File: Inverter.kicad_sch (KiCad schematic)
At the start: 45 parts, among them Q2 BSC022N04LSATMA1, Q3 BSC022N04LSATMA1, Q4 BSC022N04LSATMA1, Q5 BSC022N04LSATMA1, Q6 BSC022N04LSATMA1, Q7 BSC022N04LSATMA1, U4 TMC6140, U5 TSC2011, U6 TSC2011

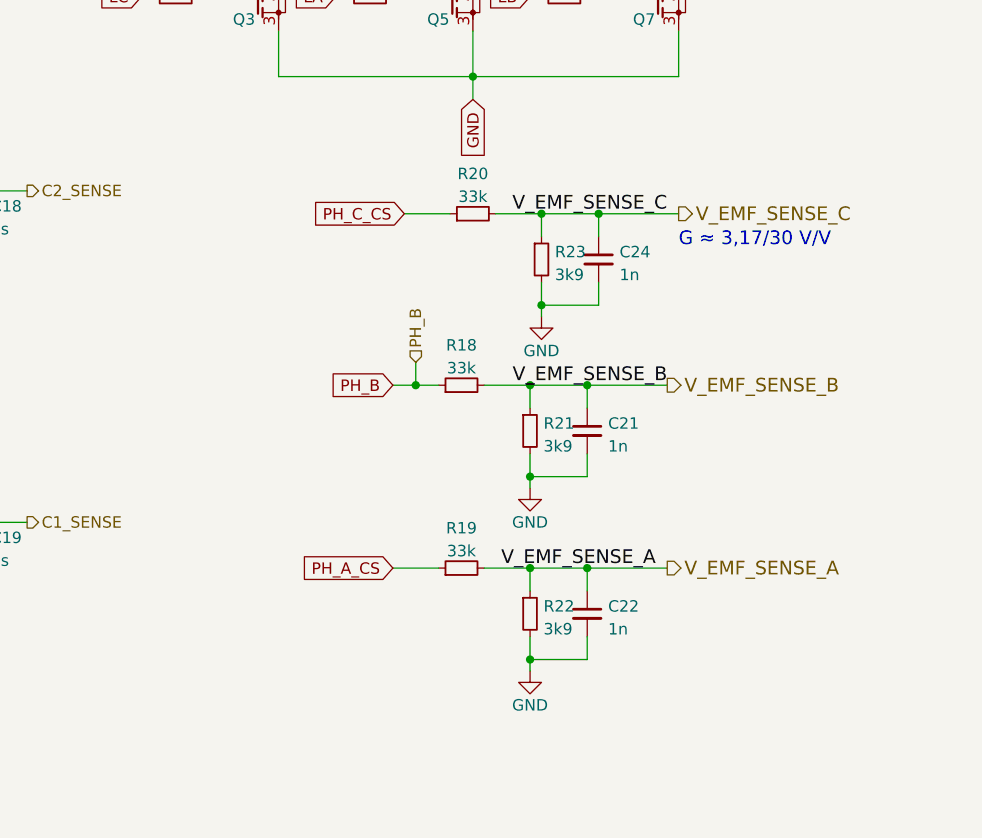
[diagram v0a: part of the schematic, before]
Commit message: layout
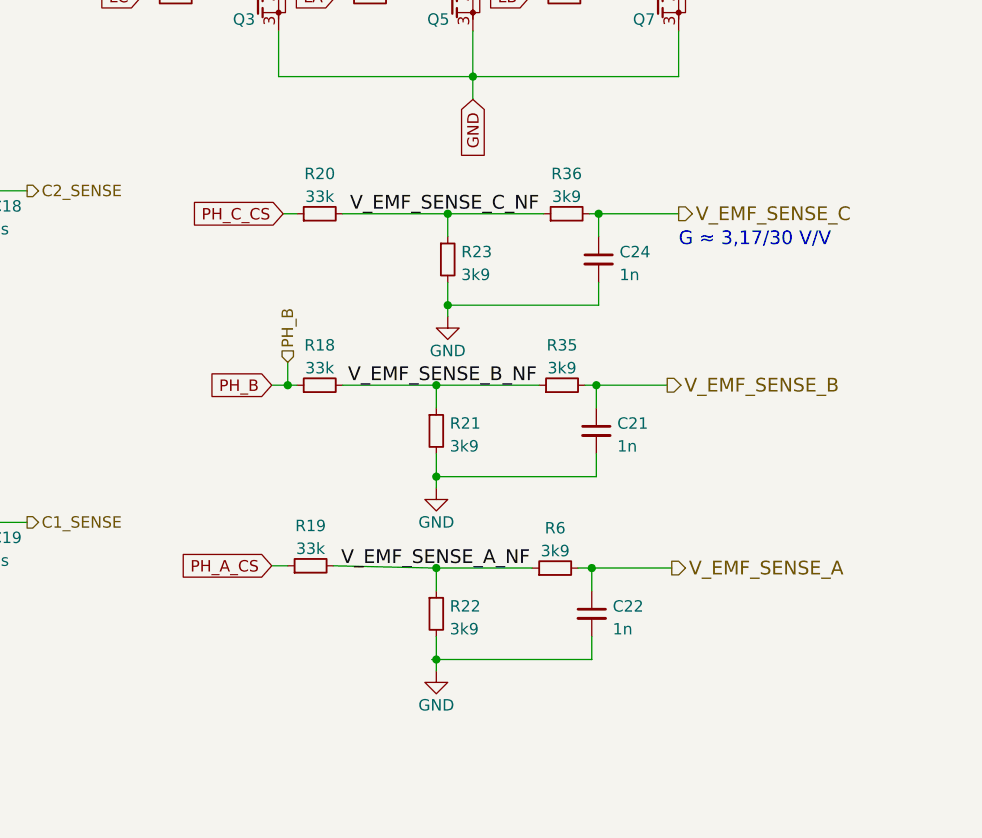
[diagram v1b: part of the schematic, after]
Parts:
- added R35, R36, R6: 3k9, Resistor_SMD:R_0603_1608Metric, symbol Device:R_Small
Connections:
- net V_EMF_SENSE_A: now also R6.2; no longer R19.2, R22.1
- net V_EMF_SENSE_B: now also R35.2; no longer R18.2, R21.1
- net V_EMF_SENSE_C: now also R36.2; no longer R20.2, R23.1
- new net V_EMF_SENSE_A_NF: R19.2, R22.1, R6.1
- new net V_EMF_SENSE_B_NF: R18.2, R21.1, R35.1
- new net V_EMF_SENSE_C_NF: R20.2, R23.1, R36.1
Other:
- moved on the sheet: C21, C22, R18, R19, R20, R21, R22, R23
